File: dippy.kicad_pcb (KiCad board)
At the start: 2 copper layers, 41.7 x 70.1 mm, 20 parts, among them J1 Conn_01x02_Female, J2 Screw_Terminal_01x03, J3 Screw_Terminal_01x04, U1 ATmega328P-PU, U2 RFM95W-915S2, U3 MCP1700-3302E_SOT23, Y1 Crystal_GND2

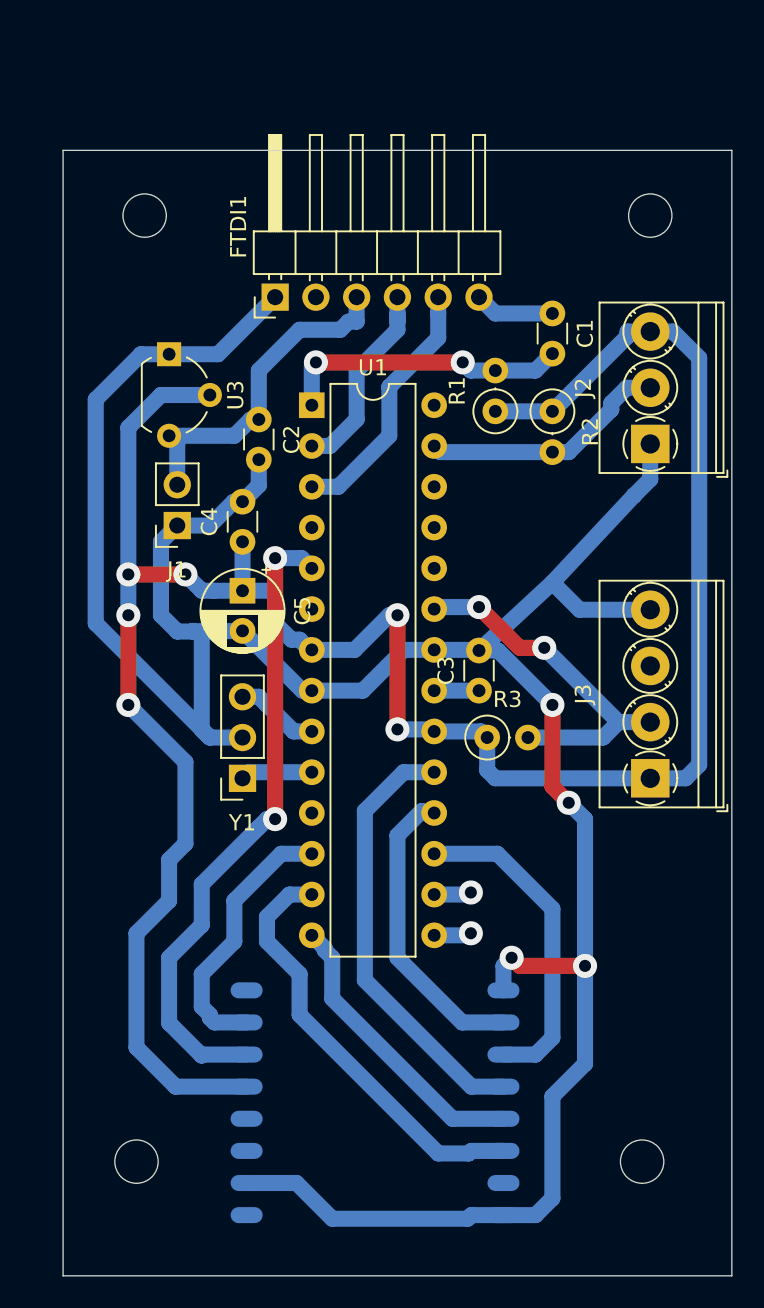
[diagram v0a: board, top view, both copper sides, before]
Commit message: update
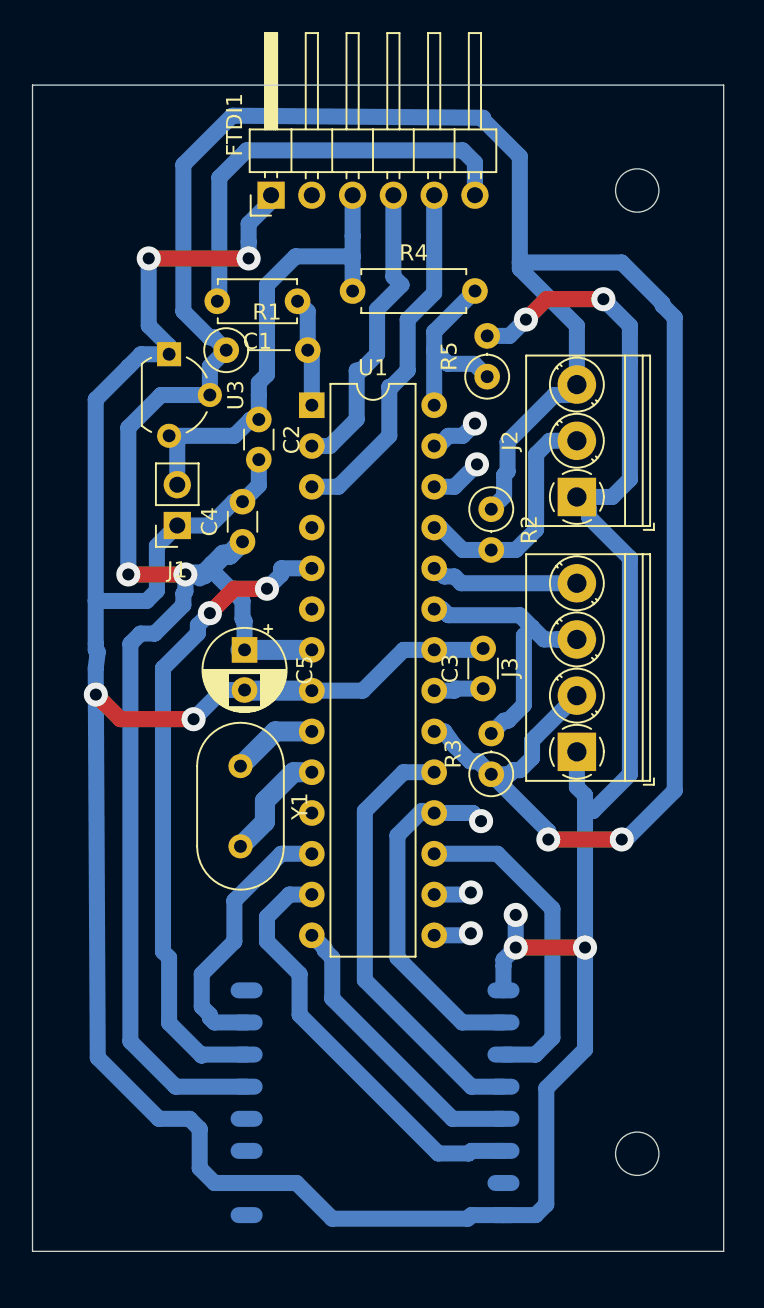
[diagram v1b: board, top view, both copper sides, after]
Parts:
- removed H1, H3: MountingHole, MountingHole:MountingHole_2.7mm_M2.5
- added R4: 100K, Resistor_THT:R_Axial_DIN0207_L6.3mm_D2.5mm_P7.62mm_Horizontal, F.Cu at (128.3, 72.3)
- added R5: 100K, Resistor_THT:R_Axial_DIN0207_L6.3mm_D2.5mm_P2.54mm_Vertical, F.Cu at (136.7, 77.6)
- C1: footprint Capacitor_THT:C_Disc_D3.0mm_W1.6mm_P2.50mm -> Capacitor_THT:C_Disc_D4.7mm_W2.5mm_P5.00mm
- R1: footprint Resistor_THT:R_Axial_DIN0207_L6.3mm_D2.5mm_P2.54mm_Vertical -> Resistor_THT:R_Axial_DIN0207_L6.3mm_D2.5mm_P5.08mm_Vertical
- U1: value ATmega328P-PU -> ATmega328P-PU-C
- Y1: value Crystal_GND2 -> Crystal; footprint Connector_PinSocket_2.54mm:PinSocket_1x03_P2.54mm_Vertical -> Crystal:Resonator-2Pin_W10.0mm_H5.0mm
- moved R1 17.2 mm to (120.4, 75.9), turned to 0 degrees
- moved C1 15.9 mm to (124.8, 72.9), turned to 180 degrees
- moved R2 7.19 mm to (136.9, 85.9)
- moved FTDI1 6.36 mm to (123.2, 66.3)
- moved J2 5.64 mm to (142.2, 85.1)
- moved J3 4.86 mm to (142.2, 101.0)
- moved C5 3.69 mm to (121.5, 94.6)
- moved R3 2.30 mm to (136.9, 102.4), turned to 90 degrees
- moved H2 1.76 mm to (146.0, 66.0)
- moved Y1 0.77 mm to (121.3, 101.9), turned to 270 degrees
- moved H4 0.58 mm to (146.0, 126.0)
- moved C3 0.28 mm to (136.4, 97.0)
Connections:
- FTDI1 pad 6: Net-(C1-Pad1) -> Net-(C1-Pad2)
- J2 pad 2: A4 -> A2
- J3 pad 1: VCC -> GND
- J3 pad 2: A0 -> VCC
- J3 pad 3: (no net) -> A0
- J3 pad 4: GND -> A1
- R1 pad 2: Net-(C1-Pad2) -> Net-(C1-Pad1)
- R2 pad 2: A4 -> A2
- U1 pad 1: Net-(C1-Pad2) -> Net-(C1-Pad1)
- U1 pad 24: (no net) -> A1
- U1 pad 25: (no net) -> A2
- U1 pad 27: A4 -> (no net)
- U1 pad 28: (no net) -> A5
- Y1 pad 1: Net-(U1-Pad10) -> Net-(U1-Pad9)
- Y1 pad 2: GND -> Net-(U1-Pad10)
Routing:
- net VCC: track 148.2 -> 207.1 mm, vias 6 -> 4
- net GND: track 173.3 -> 226.8 mm, vias 4 -> 9
- net A4: track 15.5 -> 0.00 mm
- net A2: track 0.00 -> 15.0 mm
- net A5: track 0.00 -> 12.1 mm
- net A1: track 0.00 -> 9.28 mm
- net Net-(C1-Pad2): track 18.2 -> 26.9 mm, vias 2 -> 0
- net VIN: track 21.2 -> 29.9 mm
- net (no net): track 4.68 -> 11.0 mm, vias 2 -> 4
- net TX0: track 16.0 -> 22.4 mm
- net RX0: track 12.7 -> 19.0 mm
- net A0: track 22.5 -> 18.9 mm, vias 2 -> 0
- net MISO: track 18.9 -> 22.0 mm, vias 0 -> 1
- net Net-(U1-Pad10): track 4.48 -> 7.12 mm
- net Net-(C1-Pad1): track 4.99 -> 6.85 mm
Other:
- board size 41.7 x 70.1 mm -> 43.1 x 72.6 mm

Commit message: update
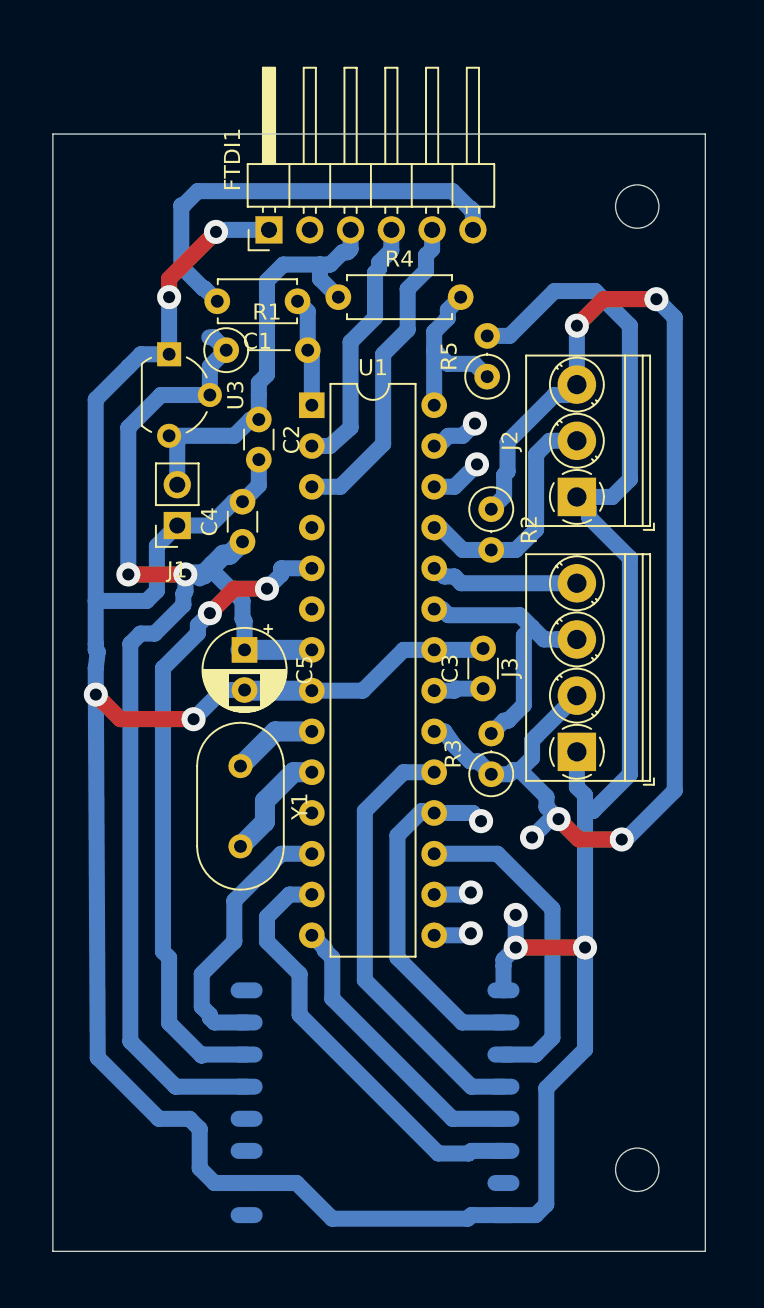
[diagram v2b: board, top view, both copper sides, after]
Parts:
- moved FTDI1 2.16 mm to (123.1, 68.5)
- moved H2 1.00 mm to (146.0, 67.0)
- moved H4 1.00 mm to (146.0, 127.0)
- moved R4 0.97 mm to (127.4, 72.6)
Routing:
- net VCC: track 207.1 -> 157.0 mm, vias 4 -> 7
- net GND: track 226.8 -> 222.7 mm, vias 9 -> 7
- net RX0: track 19.0 -> 16.2 mm
- net TX0: track 22.4 -> 20.1 mm
- net VIN: track 29.9 -> 28.0 mm
- net A5: track 12.1 -> 11.4 mm
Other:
- board size 43.1 x 72.6 mm -> 40.6 x 69.6 mm
